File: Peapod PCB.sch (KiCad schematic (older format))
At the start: 2 parts

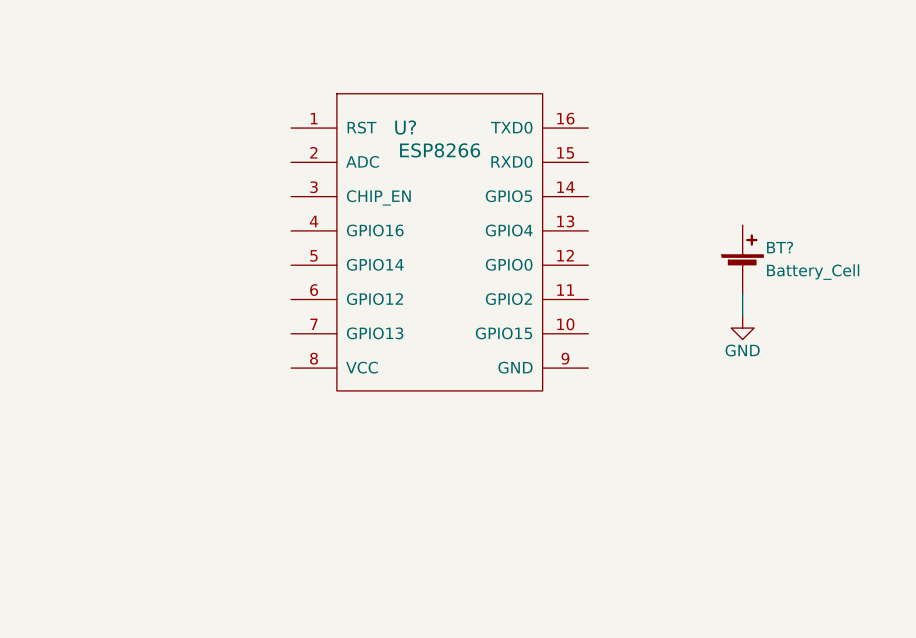
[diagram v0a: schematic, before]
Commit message: finished schematic
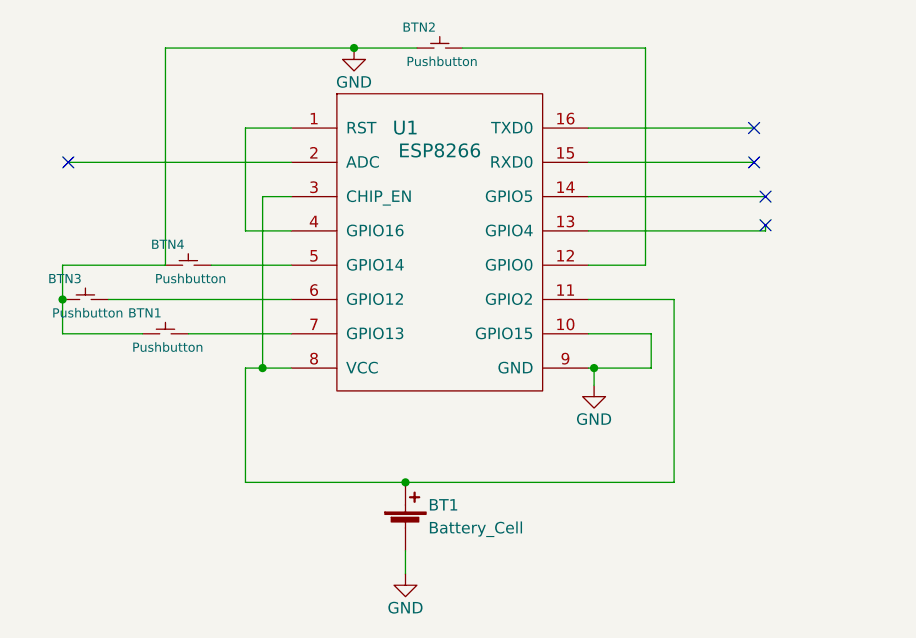
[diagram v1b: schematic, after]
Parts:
- added BTN1, BTN2, BTN3, BTN4: Pushbutton, symbol Pushbutton
- gave numbers to parts that had none: 2
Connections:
- net GND: now also U1.10 (GPIO15), U1.9 (GND), BTN1.~, BTN2.~, BTN3.~, BTN4.~
- net at U1.1 (RST): now also U1.4 (GPIO16)
- net at U1.11 (GPIO2): now also BT1.1 (+), U1.3 (CHIP_EN), U1.8 (VCC)
- net at U1.12 (GPIO0): now also BTN2.~
- net at U1.5 (GPIO14): now also BTN4.~
- net at U1.6 (GPIO12): now also BTN3.~
- net at U1.7 (GPIO13): now also BTN1.~
- no-connect marks 0 -> 5
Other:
- moved on the sheet: BT1
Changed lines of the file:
@@
 LIBS:valves
 LIBS:esp8266
+LIBS:pushbutton
+LIBS:Peapod PCB-cache
 EELAYER 25 0
 EELAYER END
@@
 $EndDescr
 $Comp
-L ESP8266 U?
+L ESP8266 U1
 U 1 1 59932095
 P 5925 3275
-F 0 "U?" H 5825 3675 60  0000 C CNN
+F 0 "U1" H 5825 3675 60  0000 C CNN
 F 1 "ESP8266" H 5975 3575 60  0000 C CNN
 F 2 "" H 5925 3275 60  0001 C CNN
@@
 $EndComp
 $Comp
-L Battery_Cell BT?
+L Battery_Cell BT1
 U 1 1 599321E0
-P 7300 3500
-F 0 "BT?" H 7400 3600 50  0000 L CNN
-F 1 "Battery_Cell" H 7400 3500 50  0000 L CNN
-F 2 "" V 7300 3560 50  0001 C CNN
-F 3 "" V 7300 3560 50  0001 C CNN
-	1    7300 3500
-	1    0    0    -1
-$EndComp
-$Comp
-L GND #PWR?
+P 5825 4625
+F 0 "BT1" H 5925 4725 50  0000 L CNN
+F 1 "Battery_Cell" H 5925 4625 50  0000 L CNN
+F 2 "" V 5825 4685 50  0001 C CNN
+F 3 "" V 5825 4685 50  0001 C CNN
+	1    5825 4625
+	1    0    0    -1
+$EndComp
+$Comp
+L GND #PWR01
 U 1 1 59932223
-P 7300 3700
-F 0 "#PWR?" H 7300 3450 50  0001 C CNN
-F 1 "GND" H 7300 3550 50  0000 C CNN
-F 2 "" H 7300 3700 50  0001 C CNN
-F 3 "" H 7300 3700 50  0001 C CNN
-	1    7300 3700
-	1    0    0    -1
-$EndComp
-Wire Wire Line
-	7300 3600 7300 3700
+P 5825 4825
+F 0 "#PWR01" H 5825 4575 50  0001 C CNN
+F 1 "GND" H 5825 4675 50  0000 C CNN
+F 2 "" H 5825 4825 50  0001 C CNN
+F 3 "" H 5825 4825 50  0001 C CNN
+	1    5825 4825
+	1    0    0    -1
+$EndComp
+$Comp
+L GND #PWR02
+U 1 1 59932907
+P 6650 4000
+F 0 "#PWR02" H 6650 3750 50  0001 C CNN
+F 1 "GND" H 6650 3850 50  0000 C CNN
+F 2 "" H 6650 4000 50  0001 C CNN
+F 3 "" H 6650 4000 50  0001 C CNN
+	1    6650 4000
+	1    0    0    -1
+$EndComp
+$Comp
+L Pushbutton BTN2
+U 1 1 59933153
+P 5975 2525
+F 0 "BTN2" H 5885 2615 40  0000 C CNN
+F 1 "Pushbutton" H 5985 2465 40  0000 C CNN
+F 2 "" H 5675 2125 60  0001 C CNN
+F 3 "" H 5675 2125 60  0001 C CNN
+	1    5975 2525
+	1    0    0    -1
+$EndComp
+$Comp
+L GND #PWR03
+U 1 1 599331DB
+P 5600 2525
+F 0 "#PWR03" H 5600 2275 50  0001 C CNN
+F 1 "GND" H 5600 2375 50  0000 C CNN
+F 2 "" H 5600 2525 50  0001 C CNN
+F 3 "" H 5600 2525 50  0001 C CNN
+	1    5600 2525
+	1    0    0    -1
+$EndComp
+$Comp
+L Pushbutton BTN1
+U 1 1 5993320C
+P 4775 3775
+F 0 "BTN1" H 4685 3865 40  0000 C CNN
+F 1 "Pushbutton" H 4785 3715 40  0000 C CNN
+F 2 "" H 4475 3375 60  0001 C CNN
+F 3 "" H 4475 3375 60  0001 C CNN
+	1    4775 3775
+	1    0    0    -1
+$EndComp
+$Comp
+L Pushbutton BTN3
+U 1 1 599332EE
+P 4425 3625
+F 0 "BTN3" H 4335 3715 40  0000 C CNN
+F 1 "Pushbutton" H 4435 3565 40  0000 C CNN
+F 2 "" H 4125 3225 60  0001 C CNN
+F 3 "" H 4125 3225 60  0001 C CNN
+	1    4425 3625
+	1    0    0    -1
+$EndComp
+$Comp
+L Pushbutton BTN4
+U 1 1 5993333F
+P 4875 3475
+F 0 "BTN4" H 4785 3565 40  0000 C CNN
+F 1 "Pushbutton" H 4885 3415 40  0000 C CNN
+F 2 "" H 4575 3075 60  0001 C CNN
+F 3 "" H 4575 3075 60  0001 C CNN
+	1    4875 3475
+	1    0    0    -1
+$EndComp
+NoConn ~ 7400 3175
+NoConn ~ 7400 3300
+NoConn ~ 7350 2875
+Wire Wire Line
+	5825 4725 5825 4825
+Wire Wire Line
+	5125 4425 5825 4425
+Wire Wire Line
+	5825 4425 7000 4425
+Wire Wire Line
+	5125 4425 5125 3925
+Wire Wire Line
+	5125 3925 5200 3925
+Wire Wire Line
+	5200 3925 5325 3925
+Wire Wire Line
+	6650 4000 6650 3925
+Wire Wire Line
+	6625 3925 6650 3925
+Wire Wire Line
+	6650 3925 6900 3925
+Wire Wire Line
+	6625 3775 6900 3775
+Wire Wire Line
+	6900 3775 6900 3925
+Connection ~ 6650 3925
+Wire Wire Line
+	7000 4425 7000 3625
+Wire Wire Line
+	7000 3625 6625 3625
+Connection ~ 5825 4425
+Wire Wire Line
+	6625 3475 6875 3475
+Wire Wire Line
+	6875 3475 6875 2525
+Wire Wire Line
+	6875 2525 6075 2525
+Wire Wire Line
+	4775 2525 5600 2525
+Wire Wire Line
+	5600 2525 5875 2525
+Wire Wire Line
+	5325 3175 5200 3175
+Wire Wire Line
+	5200 3175 5200 3925
+Connection ~ 5200 3925
+Wire Wire Line
+	5325 2875 5125 2875
+Wire Wire Line
+	5125 2875 5125 3325
+Wire Wire Line
+	5125 3325 5325 3325
+Wire Wire Line
+	5325 3775 4875 3775
+Wire Wire Line
+	5325 3475 4975 3475
+Wire Wire Line
+	5325 3625 4525 3625
+Wire Wire Line
+	4325 3775 4675 3775
+Wire Wire Line
+	4325 3475 4325 3625
+Wire Wire Line
+	4325 3625 4325 3775
+Wire Wire Line
+	4325 3475 4775 3475
+Connection ~ 4325 3625
+Wire Wire Line
+	4775 3475 4775 2525
+Connection ~ 5600 2525
+Wire Wire Line
+	6625 3175 7400 3175
+Wire Wire Line
+	6625 3325 7400 3325
+Wire Wire Line
+	7400 3325 7400 3300
+Wire Wire Line
+	6625 2875 7350 2875
+Wire Wire Line
+	6625 3025 7350 3025
+NoConn ~ 7350 3025
+Wire Wire Line
+	5325 3025 4350 3025
+NoConn ~ 4350 3025
 $EndSCHEMATC

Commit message: updated schematic
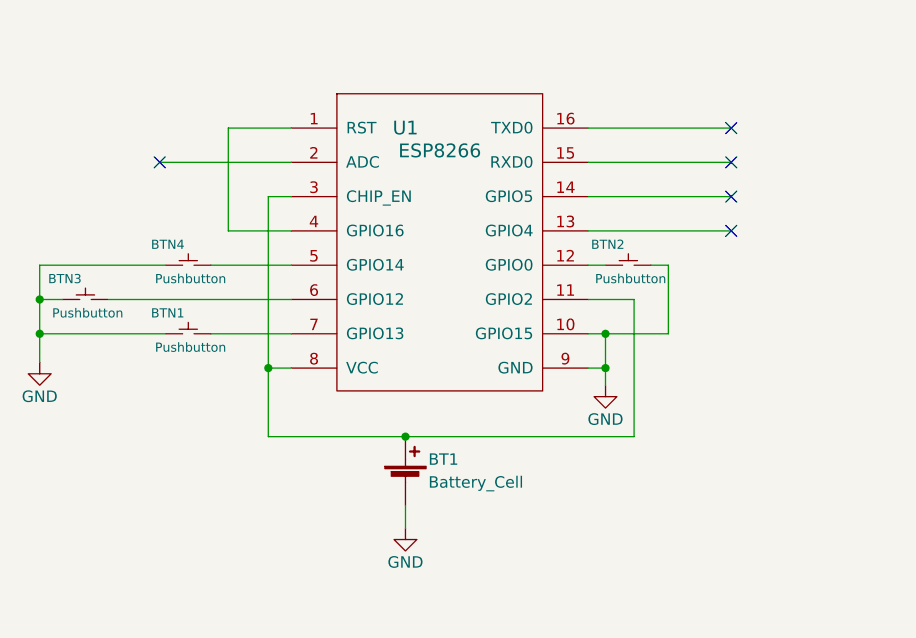
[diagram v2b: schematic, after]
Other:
- moved on the sheet: BT1, BTN1, BTN2
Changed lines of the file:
@@
 L Battery_Cell BT1
 U 1 1 599321E0
-P 5825 4625
-F 0 "BT1" H 5925 4725 50  0000 L CNN
-F 1 "Battery_Cell" H 5925 4625 50  0000 L CNN
-F 2 "" V 5825 4685 50  0001 C CNN
-F 3 "" V 5825 4685 50  0001 C CNN
-	1    5825 4625
+P 5825 4425
+F 0 "BT1" H 5925 4525 50  0000 L CNN
+F 1 "Battery_Cell" H 5925 4425 50  0000 L CNN
+F 2 "" V 5825 4485 50  0001 C CNN
+F 3 "" V 5825 4485 50  0001 C CNN
+	1    5825 4425
 	1    0    0    -1
 $EndComp
@@
 L GND #PWR01
 U 1 1 59932223
-P 5825 4825
-F 0 "#PWR01" H 5825 4575 50  0001 C CNN
-F 1 "GND" H 5825 4675 50  0000 C CNN
-F 2 "" H 5825 4825 50  0001 C CNN
-F 3 "" H 5825 4825 50  0001 C CNN
-	1    5825 4825
+P 5825 4625
+F 0 "#PWR01" H 5825 4375 50  0001 C CNN
+F 1 "GND" H 5825 4475 50  0000 C CNN
+F 2 "" H 5825 4625 50  0001 C CNN
+F 3 "" H 5825 4625 50  0001 C CNN
+	1    5825 4625
 	1    0    0    -1
 $EndComp
@@
 L GND #PWR02
 U 1 1 59932907
-P 6650 4000
-F 0 "#PWR02" H 6650 3750 50  0001 C CNN
-F 1 "GND" H 6650 3850 50  0000 C CNN
-F 2 "" H 6650 4000 50  0001 C CNN
-F 3 "" H 6650 4000 50  0001 C CNN
-	1    6650 4000
+P 6700 4000
+F 0 "#PWR02" H 6700 3750 50  0001 C CNN
+F 1 "GND" H 6700 3850 50  0000 C CNN
+F 2 "" H 6700 4000 50  0001 C CNN
+F 3 "" H 6700 4000 50  0001 C CNN
+	1    6700 4000
 	1    0    0    -1
 $EndComp
@@
 L Pushbutton BTN2
 U 1 1 59933153
-P 5975 2525
-F 0 "BTN2" H 5885 2615 40  0000 C CNN
-F 1 "Pushbutton" H 5985 2465 40  0000 C CNN
-F 2 "" H 5675 2125 60  0001 C CNN
-F 3 "" H 5675 2125 60  0001 C CNN
-	1    5975 2525
-	1    0    0    -1
-$EndComp
-$Comp
-L GND #PWR03
-U 1 1 599331DB
-P 5600 2525
-F 0 "#PWR03" H 5600 2275 50  0001 C CNN
-F 1 "GND" H 5600 2375 50  0000 C CNN
-F 2 "" H 5600 2525 50  0001 C CNN
-F 3 "" H 5600 2525 50  0001 C CNN
-	1    5600 2525
+P 6800 3475
+F 0 "BTN2" H 6710 3565 40  0000 C CNN
+F 1 "Pushbutton" H 6810 3415 40  0000 C CNN
+F 2 "" H 6500 3075 60  0001 C CNN
+F 3 "" H 6500 3075 60  0001 C CNN
+	1    6800 3475
 	1    0    0    -1
 $EndComp
@@
 L Pushbutton BTN1
 U 1 1 5993320C
-P 4775 3775
-F 0 "BTN1" H 4685 3865 40  0000 C CNN
-F 1 "Pushbutton" H 4785 3715 40  0000 C CNN
-F 2 "" H 4475 3375 60  0001 C CNN
-F 3 "" H 4475 3375 60  0001 C CNN
-	1    4775 3775
+P 4875 3775
+F 0 "BTN1" H 4785 3865 40  0000 C CNN
+F 1 "Pushbutton" H 4885 3715 40  0000 C CNN
+F 2 "" H 4575 3375 60  0001 C CNN
+F 3 "" H 4575 3375 60  0001 C CNN
+	1    4875 3775
 	1    0    0    -1
 $EndComp
@@
 	1    0    0    -1
 $EndComp
-NoConn ~ 7400 3175
-NoConn ~ 7400 3300
-NoConn ~ 7350 2875
+NoConn ~ 7250 3175
+NoConn ~ 7250 3325
+NoConn ~ 7250 2875
 Wire Wire Line
-	5825 4725 5825 4825
+	5825 4525 5825 4625
 Wire Wire Line
-	5125 4425 5825 4425
+	5225 4225 5825 4225
 Wire Wire Line
-	5825 4425 7000 4425
+	5825 4225 6825 4225
 Wire Wire Line
-	5125 4425 5125 3925
+	5225 3175 5225 3925
 Wire Wire Line
-	5125 3925 5200 3925
+	5225 3925 5225 4225
 Wire Wire Line
-	5200 3925 5325 3925
+	5225 3925 5325 3925
 Wire Wire Line
-	6650 4000 6650 3925
+	6700 3775 6700 3925
 Wire Wire Line
-	6625 3925 6650 3925
+	6700 3925 6700 4000
 Wire Wire Line
-	6650 3925 6900 3925
+	6700 3925 6625 3925
 Wire Wire Line
-	6625 3775 6900 3775
+	6625 3775 6700 3775
 Wire Wire Line
-	6900 3775 6900 3925
-Connection ~ 6650 3925
+	6700 3775 6975 3775
+Connection ~ 6700 3925
 Wire Wire Line
-	7000 4425 7000 3625
+	6825 4225 6825 3625
 Wire Wire Line
-	7000 3625 6625 3625
-Connection ~ 5825 4425
+	6825 3625 6625 3625
+Connection ~ 5825 4225
 Wire Wire Line
-	6625 3475 6875 3475
+	5325 3175 5225 3175
+Connection ~ 5225 3925
 Wire Wire Line
-	6875 3475 6875 2525
+	5325 2875 5050 2875
 Wire Wire Line
-	6875 2525 6075 2525
+	5050 2875 5050 3325
 Wire Wire Line
-	4775 2525 5600 2525
+	5050 3325 5325 3325
 Wire Wire Line
-	5600 2525 5875 2525
-Wire Wire Line
-	5325 3175 5200 3175
-Wire Wire Line
-	5200 3175 5200 3925
-Connection ~ 5200 3925
-Wire Wire Line
-	5325 2875 5125 2875
-Wire Wire Line
-	5125 2875 5125 3325
-Wire Wire Line
-	5125 3325 5325 3325
-Wire Wire Line
-	5325 3775 4875 3775
+	5325 3775 4975 3775
 Wire Wire Line
 	5325 3475 4975 3475
@@
 	5325 3625 4525 3625
 Wire Wire Line
-	4325 3775 4675 3775
+	4225 3775 4775 3775
 Wire Wire Line
-	4325 3475 4325 3625
+	4225 3475 4225 3625
 Wire Wire Line
-	4325 3625 4325 3775
+	4225 3625 4225 3775
 Wire Wire Line
-	4325 3475 4775 3475
-Connection ~ 4325 3625
+	4225 3775 4225 3900
+Connection ~ 4225 3625
 Wire Wire Line
-	4775 3475 4775 2525
-Connection ~ 5600 2525
+	6625 3175 7250 3175
 Wire Wire Line
-	6625 3175 7400 3175
+	6625 3325 7250 3325
 Wire Wire Line
-	6625 3325 7400 3325
+	7250 3325 7250 3325
 Wire Wire Line
-	7400 3325 7400 3300
+	6625 2875 7250 2875
 Wire Wire Line
-	6625 2875 7350 2875
+	6625 3025 7250 3025
+NoConn ~ 7250 3025
 Wire Wire Line
-	6625 3025 7350 3025
-NoConn ~ 7350 3025
+	5325 3025 4750 3025
+NoConn ~ 4750 3025
+$Comp
+L GND #PWR?
+U 1 1 5993357D
+P 4225 3900
+F 0 "#PWR?" H 4225 3650 50  0001 C CNN
+F 1 "GND" H 4225 3750 50  0000 C CNN
+F 2 "" H 4225 3900 50  0001 C CNN
+F 3 "" H 4225 3900 50  0001 C CNN
+	1    4225 3900
+	1    0    0    -1
+$EndComp
 Wire Wire Line
-	5325 3025 4350 3025
-NoConn ~ 4350 3025
+	4775 3475 4225 3475
+Connection ~ 4225 3775
+Wire Wire Line
+	4325 3625 4225 3625
+Wire Wire Line
+	6975 3775 6975 3475
+Wire Wire Line
+	6975 3475 6900 3475
+Connection ~ 6700 3775
+Wire Wire Line
+	6625 3475 6700 3475
 $EndSCHEMATC
